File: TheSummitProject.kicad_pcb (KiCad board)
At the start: 4 copper layers, 91.5 x 65 mm, 81 parts, among them IC1 STM32U5F7VJT6, J1 Cortex SWD, J4 Screen FPC, J5 Micro_SD_Card_Det1, Q1 NMOS, SW1 SW_SPDT, SW2 PWR_BTN, U1 NPM1300-CAAA-R, U2 USBLC6-2SC6, U3 USBLC6-2SC6, Y1 16Mhz, Y2 32.768Khz

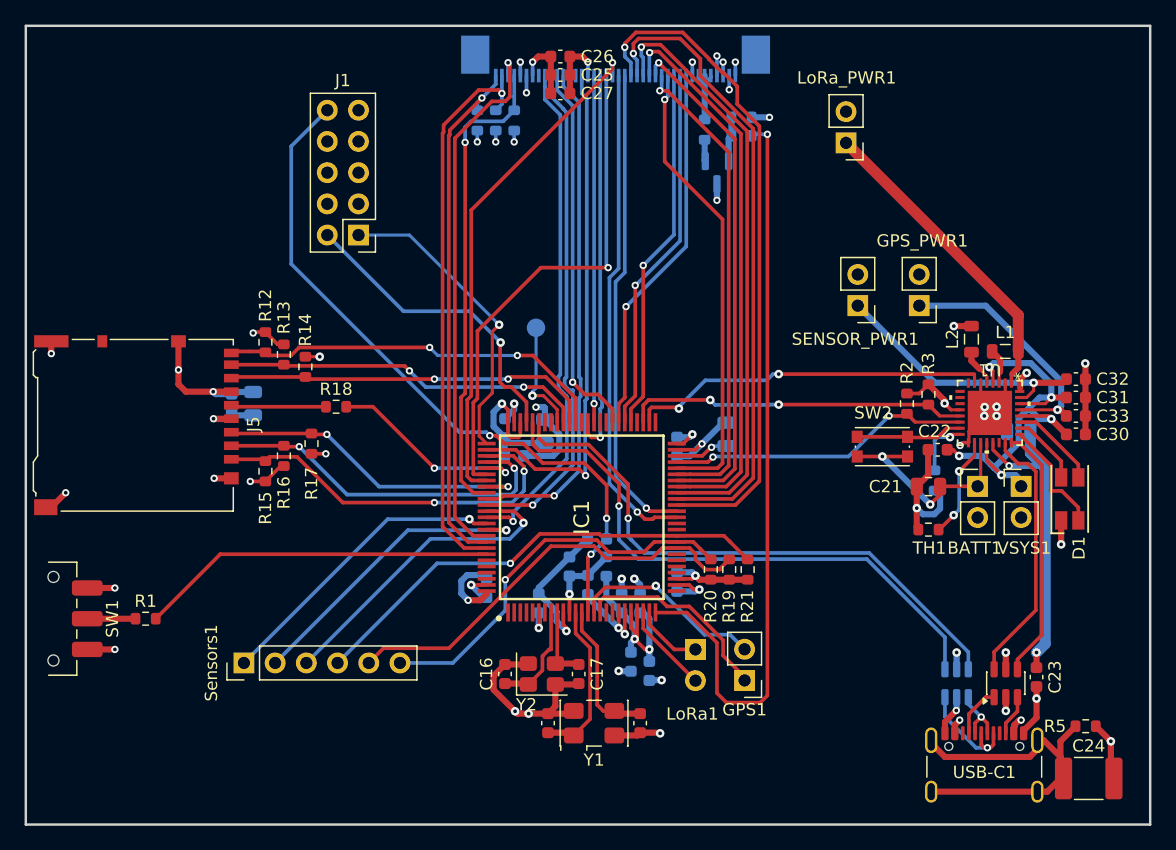
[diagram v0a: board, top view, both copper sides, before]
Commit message: DFM tested and edited
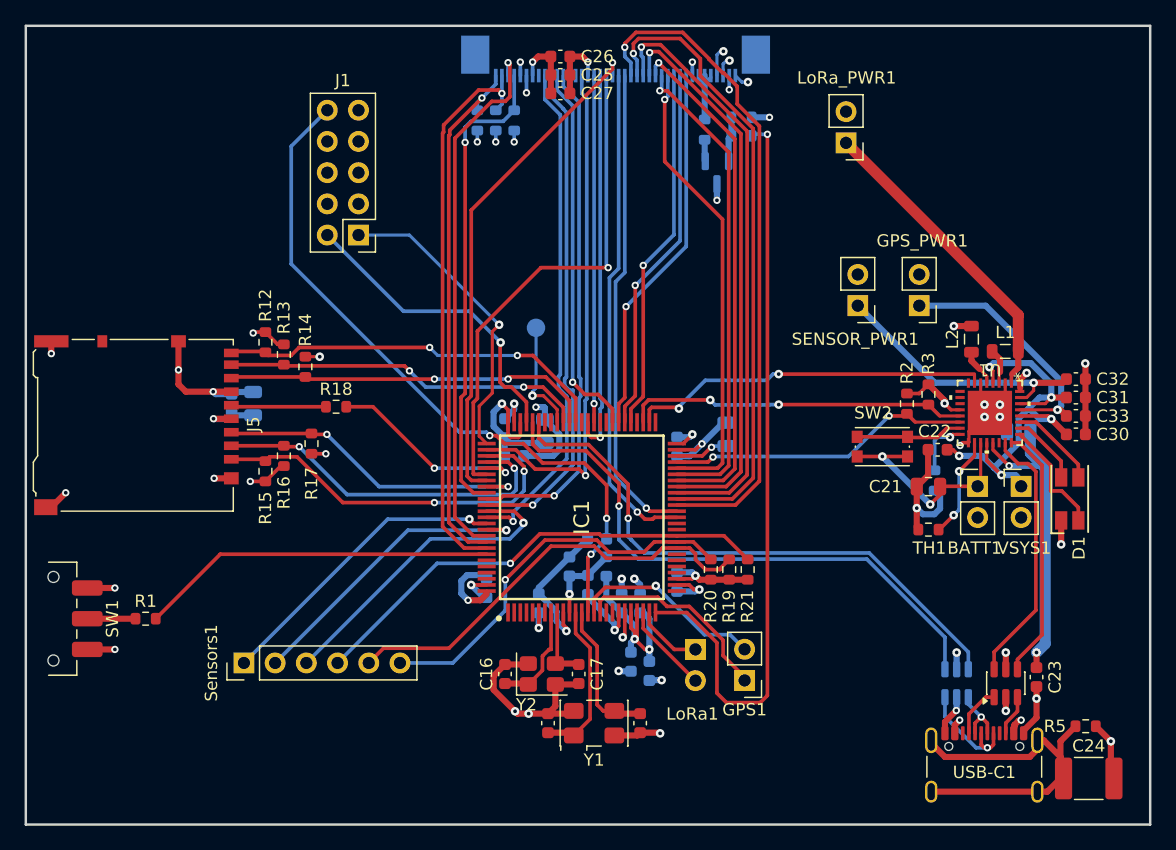
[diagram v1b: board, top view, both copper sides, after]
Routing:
- net GND: track 140.3 -> 137.9 mm
- net +3.3V: track 65.8 -> 64.4 mm
- net Net-(USB-C1-SHIELD): track 28.5 -> 27.5 mm
- net Net-(IC1-HSE_OUT): track 12.1 -> 11.5 mm
